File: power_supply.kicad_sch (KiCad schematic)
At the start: 9 parts, among them IC1 ST1PS03AQTR, Q3 AO3401A

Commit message: Added footprint for components in Schematics. Updated LED resistors
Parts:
- C13, C22: footprint (none) -> Capacitor_SMD:C_0805_2012Metric
- C30: footprint (none) -> Capacitor_SMD:C_0201_0603Metric
- F1: footprint (none) -> Fuse:Fuse_1206_3216Metric
- FB1, L3: footprint (none) -> Inductor_SMD:L_0805_2012Metric
- R6: footprint (none) -> Resistor_SMD:R_0805_2012Metric
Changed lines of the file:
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@@
     (property "Reference" "L3" (id 0) (at 144.78 128.27 90))
     (property "Value" "2u2H" (id 1) (at 144.78 130.81 90))
-    (property "Footprint" "" (id 2) (at 144.78 133.35 0)
+    (property "Footprint" "Inductor_SMD:L_0805_2012Metric" (id 2) (at 144.78 133.35 0)
       (effects (font (size 1.27 1.27)) hide)
     )
@@
       (effects (font (size 1.27 1.27)) (justify left))
     )
-    (property "Footprint" "" (id 2) (at 189.23 102.87 0)
+    (property "Footprint" "Resistor_SMD:R_0805_2012Metric" (id 2) (at 189.23 102.87 0)
       (effects (font (size 1.27 1.27)) hide)
     )
@@
       (effects (font (size 1.27 1.27)) (justify left))
     )
-    (property "Footprint" "" (id 2) (at 127 99.06 0)
+    (property "Footprint" "Capacitor_SMD:C_0805_2012Metric" (id 2) (at 127 99.06 0)
       (effects (font (size 1.27 1.27)) hide)
     )
@@
     (property "Reference" "FB1" (id 0) (at 119.3419 85.09 90))
     (property "Value" "600@100MHz" (id 1) (at 123.19 87.63 90))
-    (property "Footprint" "" (id 2) (at 119.38 93.218 90)
+    (property "Footprint" "Inductor_SMD:L_0805_2012Metric" (id 2) (at 119.38 93.218 90)
       (effects (font (size 1.27 1.27)) hide)
     )
@@
     (property "Reference" "F1" (id 0) (at 109.22 85.09 90))
     (property "Value" "500mA" (id 1) (at 109.22 87.63 90))
-    (property "Footprint" "" (id 2) (at 114.3 90.17 0)
+    (property "Footprint" "Fuse:Fuse_1206_3216Metric" (id 2) (at 114.3 90.17 0)
       (effects (font (size 1.27 1.27)) (justify left) hide)
     )
@@
       (effects (font (size 1.27 1.27)) (justify left))
     )
-    (property "Footprint" "" (id 2) (at 161.29 121.92 0)
+    (property "Footprint" "Capacitor_SMD:C_0201_0603Metric" (id 2) (at 161.29 121.92 0)
       (effects (font (size 1.27 1.27)) hide)
     )
@@
       (effects (font (size 1.27 1.27)) (justify left))
     )
-    (property "Footprint" "" (id 2) (at 201.93 114.3 0)
-      (effects (font (size 1.27 1.27)) hide)
-    )
+    (property "Footprint" "Capacitor_SMD:C_0805_2012Metric" (id 2) (at 201.93 114.3 0)
+      (effects (font (size 1.27 1.27)) hide)
+    )

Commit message: Added preliminary PCL layout
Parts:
- C30: footprint Capacitor_SMD:C_0201_0603Metric -> Capacitor_SMD:C_0603_1608Metric
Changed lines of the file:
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@@
       (effects (font (size 1.27 1.27)) (justify left))
     )
-    (property "Footprint" "Capacitor_SMD:C_0201_0603Metric" (id 2) (at 161.29 121.92 0)
+    (property "Footprint" "Capacitor_SMD:C_0603_1608Metric" (id 2) (at 161.29 121.92 0)
       (effects (font (size 1.27 1.27)) hide)
     )

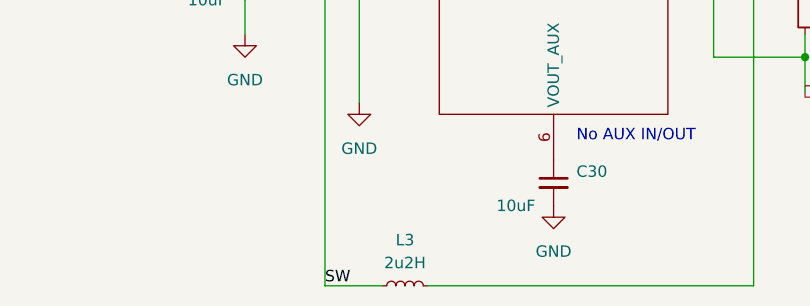
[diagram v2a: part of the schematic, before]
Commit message: Revision 1 of the board that was manufactured
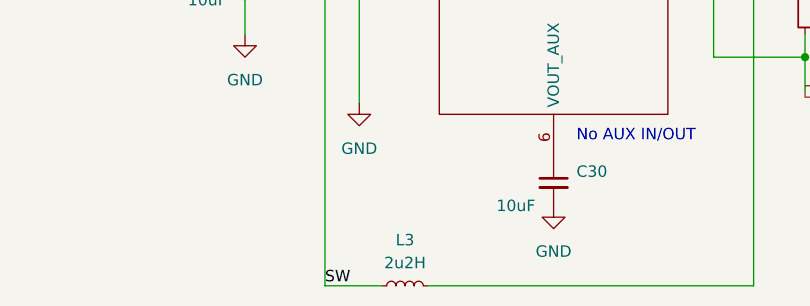
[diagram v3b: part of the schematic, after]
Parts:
- C13, C22: LCSC (none) -> C15850
- C30: LCSC (none) -> C96446
- F1: LCSC (none) -> C69688
- FB1: LCSC (none) -> C1017
- IC1: LCSC (none) -> C3187888
- L3: LCSC (none) -> C370034
- Q3: LCSC (none) -> C15127
- R6: LCSC (none) -> C441966
